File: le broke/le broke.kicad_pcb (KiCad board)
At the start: 2 copper layers, 99.7 x 75.9 mm, 37 parts, among them U1 ProMicro

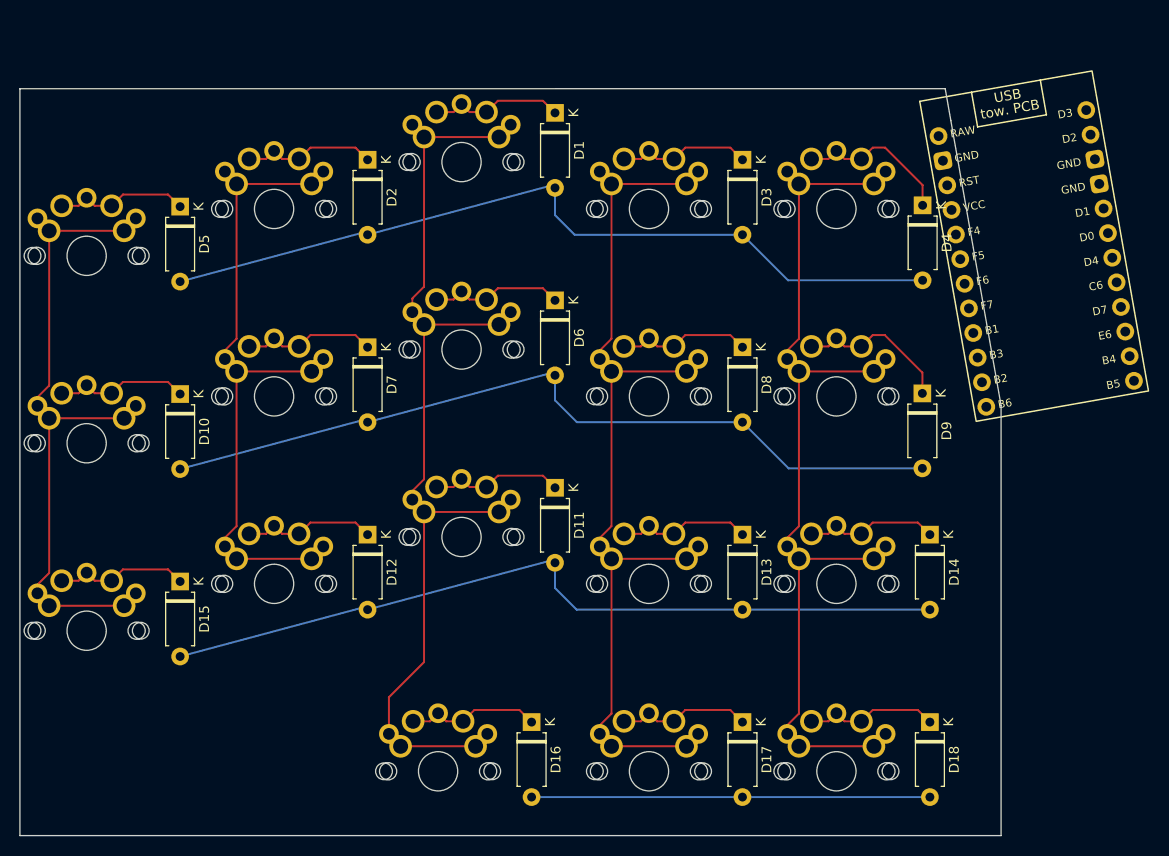
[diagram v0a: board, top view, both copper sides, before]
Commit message: did a lebroke thing idk
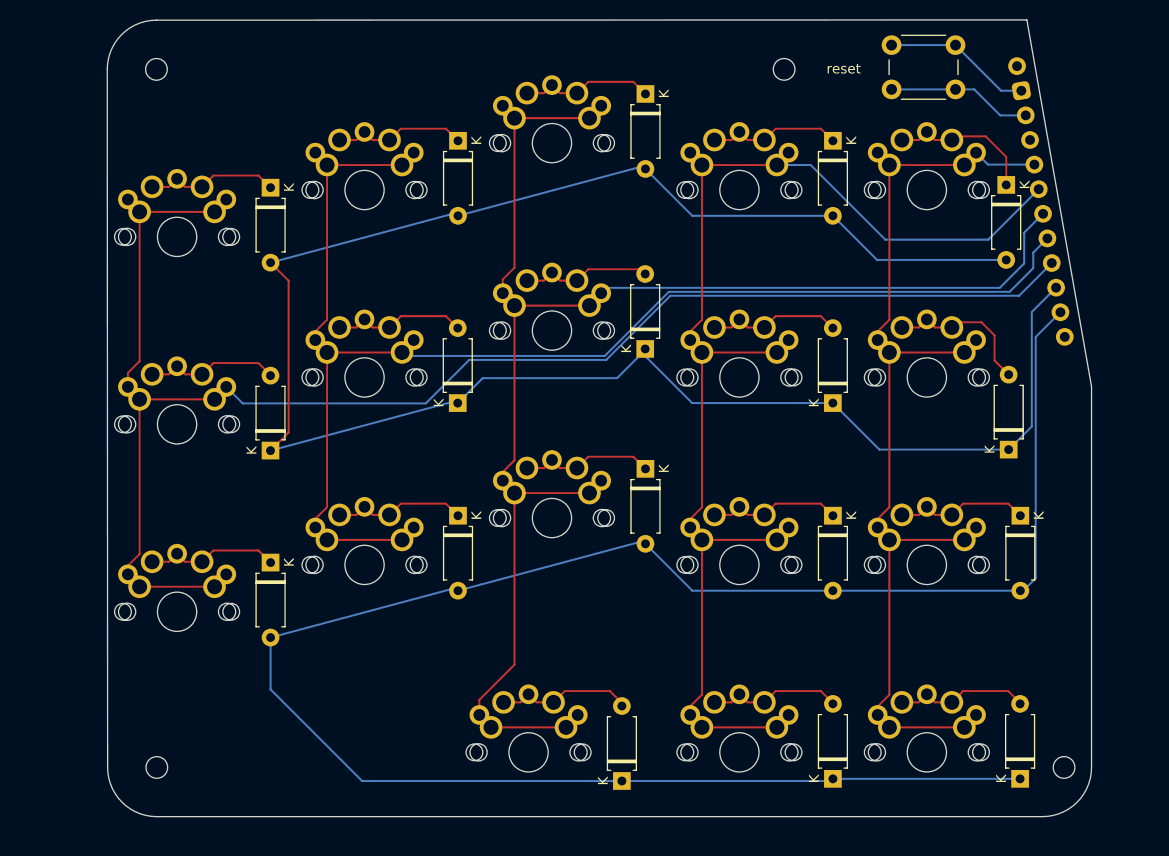
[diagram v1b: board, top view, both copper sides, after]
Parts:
- added REF**: MountingHole_2.2mm_M2, MountingHole:MountingHole_2.2mm_M2, F.Cu at (98.1, 56.1)
- added REF**: MountingHole_2.2mm_M2, MountingHole:MountingHole_2.2mm_M2, F.Cu at (190.4, 127.0)
- added REF**: MountingHole_2.2mm_M2, MountingHole:MountingHole_2.2mm_M2, F.Cu at (98.1, 127.0)
- added REF**: MountingHole_2.2mm_M2, MountingHole:MountingHole_2.2mm_M2, F.Cu at (161.9, 56.1)
- added SW1: SW_Push, Button_Switch_THT:SW_PUSH_6mm, F.Cu at (172.8, 53.6)
- moved D16 11.0 mm to (145.4, 128.4), turned to 90 degrees
- moved D17 10.9 mm to (166.9, 128.2), turned to 90 degrees
- moved D10 10.8 mm to (109.7, 94.8), turned to 90 degrees
- moved D18 10.8 mm to (185.9, 128.2), turned to 90 degrees
- moved D8 10.8 mm to (166.9, 90.0), turned to 90 degrees
- moved D7 10.8 mm to (128.7, 90.0), turned to 90 degrees
- moved U1 10.7 mm to (195.5, 68.2)
- moved D9 10.5 mm to (184.7, 94.7), turned to 90 degrees
- moved D6 10.4 mm to (147.8, 84.5), turned to 90 degrees
- moved D2 9.39 mm to (128.8, 63.3)
- moved MX5 9.39 mm to (100.2, 73.1)
- moved MX16 9.39 mm to (135.9, 125.5)
- moved MX4 9.39 mm to (176.4, 68.3)
- moved MX9 9.39 mm to (176.4, 87.4)
- moved D1 9.39 mm to (147.8, 58.5)
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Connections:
- D1 pad 2: Net-(D1-A) -> ROW0
- D10 pad 1: Net-(D10-K) -> ROW0
- D11 pad 2: Net-(D11-A) -> ROW1
- D12 pad 2: Net-(D11-A) -> ROW1
- D13 pad 2: Net-(D11-A) -> ROW1
- D14 pad 2: Net-(D11-A) -> ROW1
- D15 pad 2: Net-(D11-A) -> ROW1
- D16 pad 1: Net-(D16-K) -> ROW1
- D17 pad 1: Net-(D17-K) -> ROW1
- D17 pad 2: Net-(D16-A) -> Net-(D17-A)
- D18 pad 1: Net-(D18-K) -> ROW1
- D18 pad 2: Net-(D16-A) -> Net-(D18-A)
- D2 pad 2: Net-(D1-A) -> ROW0
- D3 pad 2: Net-(D1-A) -> ROW0
- D4 pad 2: Net-(D1-A) -> ROW0
- D5 pad 2: Net-(D1-A) -> ROW0
- D6 pad 1: Net-(D6-K) -> ROW0
- D6 pad 2: Net-(D10-A) -> Net-(D6-A)
- D7 pad 1: Net-(D7-K) -> ROW0
- D7 pad 2: Net-(D10-A) -> Net-(D7-A)
- D8 pad 1: Net-(D8-K) -> ROW0
- D8 pad 2: Net-(D10-A) -> Net-(D8-A)
- D9 pad 1: Net-(D9-K) -> ROW0
- D9 pad 2: Net-(D10-A) -> Net-(D9-A)
- MX1 pad 1: Net-(MX1-Pad1) -> COL2
- MX10 pad 1: Net-(MX10-Pad1) -> COL0
- MX10 pad 2: Net-(D10-K) -> Net-(D10-A)
- MX11 pad 1: Net-(MX1-Pad1) -> COL2
- MX12 pad 1: Net-(MX12-Pad1) -> COL1
- MX13 pad 1: Net-(MX13-Pad1) -> COL3
- MX14 pad 1: Net-(MX14-Pad1) -> COL4
- MX15 pad 1: Net-(MX10-Pad1) -> COL0
- MX16 pad 1: Net-(MX1-Pad1) -> COL2
- MX16 pad 2: Net-(D16-K) -> Net-(D16-A)
- MX17 pad 1: Net-(MX13-Pad1) -> COL3
- MX17 pad 2: Net-(D17-K) -> Net-(D17-A)
- MX18 pad 1: Net-(MX14-Pad1) -> COL4
- MX18 pad 2: Net-(D18-K) -> Net-(D18-A)
- MX2 pad 1: Net-(MX12-Pad1) -> COL1
- MX3 pad 1: Net-(MX13-Pad1) -> COL3
- MX4 pad 1: Net-(MX14-Pad1) -> COL4
- MX5 pad 1: Net-(MX10-Pad1) -> COL0
- MX6 pad 1: Net-(MX1-Pad1) -> COL2
- MX6 pad 2: Net-(D6-K) -> Net-(D6-A)
- MX7 pad 1: Net-(MX12-Pad1) -> COL1
- MX7 pad 2: Net-(D7-K) -> Net-(D7-A)
- MX8 pad 1: Net-(MX13-Pad1) -> COL3
- MX8 pad 2: Net-(D8-K) -> Net-(D8-A)
- MX9 pad 1: Net-(MX14-Pad1) -> COL4
- MX9 pad 2: Net-(D9-K) -> Net-(D9-A)
- U1 pad 14: unconnected-(U1-GND-Pad14) -> Net-(SW1-Pad1)
- U1 pad 15: unconnected-(U1-RST-Pad15) -> Net-(U1-RST)
- U1 pad 17: unconnected-(U1-F4-Pad17) -> COL4
- U1 pad 18: unconnected-(U1-F5-Pad18) -> COL3
- U1 pad 19: unconnected-(U1-F6-Pad19) -> COL2
- U1 pad 20: unconnected-(U1-F7-Pad20) -> COL1
- U1 pad 21: unconnected-(U1-B1-Pad21) -> COL0
- U1 pad 22: unconnected-(U1-B3-Pad22) -> ROW0
- U1 pad 23: unconnected-(U1-B2-Pad23) -> ROW1
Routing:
- net ROW0: track 0.00 -> 202.0 mm
- net ROW1: track 0.00 -> 195.2 mm
- net COL0: track 0.00 -> 149.9 mm
- net COL2: track 0.00 -> 142.9 mm
- net COL1: track 0.00 -> 131.0 mm
- net COL3: track 0.00 -> 117.2 mm
- net COL4: track 0.00 -> 91.8 mm
- net Net-(MX1-Pad1): track 91.1 -> 0.00 mm
- net Net-(MX13-Pad1): track 85.3 -> 0.00 mm
- net Net-(MX14-Pad1): track 85.3 -> 0.00 mm
- net Net-(D1-A): track 82.4 -> 0.00 mm
- net Net-(D11-A): track 81.1 -> 0.00 mm
- net Net-(D10-A): track 82.3 -> 13.7 mm
- net Net-(MX10-Pad1): track 59.4 -> 0.00 mm
- net Net-(MX12-Pad1): track 59.4 -> 0.00 mm
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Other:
- board size 99.7 x 75.9 mm -> 100 x 81 mm
- board text added: "reset"
- board text added: "wake"
